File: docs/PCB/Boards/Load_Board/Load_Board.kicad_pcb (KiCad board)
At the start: 2 copper layers, 108.1 x 74.8 mm, 114 parts, among them J1 Conn_02x04_Odd_Even, J10 LVL_OUT_3, J11 LVL_IN_4, J12 LVL_OUT_4, J13 LVL_IN_6, J14 LVL_OUT_6, J15 LVL_IN_5, J16 LVL_OUT_5, J2 Conn_02x04_Odd_Even, J21 R_IN, J22 R_OUT, J23 SW_IN, J24 SW_OUT, J25 Divider_1, J26 Divider_2, J27 BZ_IN, J28 BZ_OUT, J29 LED_IN, J3 Conn_01x06_Pin, J30 LED_OUT, J31 CRYSTAL_IN, J32 CRYSTAL_OUT, J33 T_1, J34 T_2, J35 L_IN, J36 L_OUT, J37 C_IN, J38 C_OUT, J39 RV1, J4 Conn_01x06_Pin, J40 RV2, J41 RV3, J5 LVL_IN_2, J6 LVL_OUT_2, J7 LVL_IN_1, J8 LVL_OUT_1, J9 LVL_IN_3, Q1 BSS138, Q2 BSS138, Q3 BSS138, Q4 BSS138, Q5 BSS138, Q6 BSS138, Q7 BSS138, Q8 BSS138, SW1 Tact Switch 6x6mm / 13mm, U1 NE555P, Y1 Crystal, Y2 Crystal, Y3 Crystal

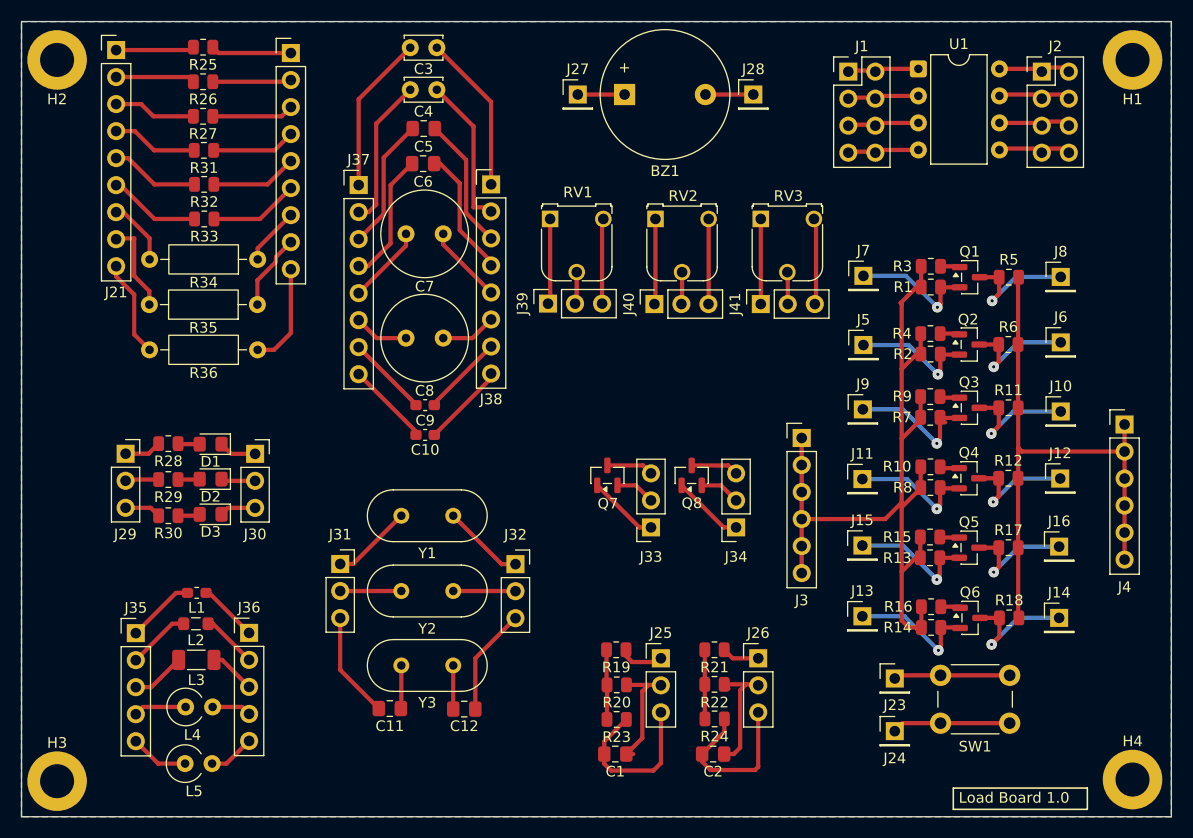
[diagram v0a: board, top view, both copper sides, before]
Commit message: Code review
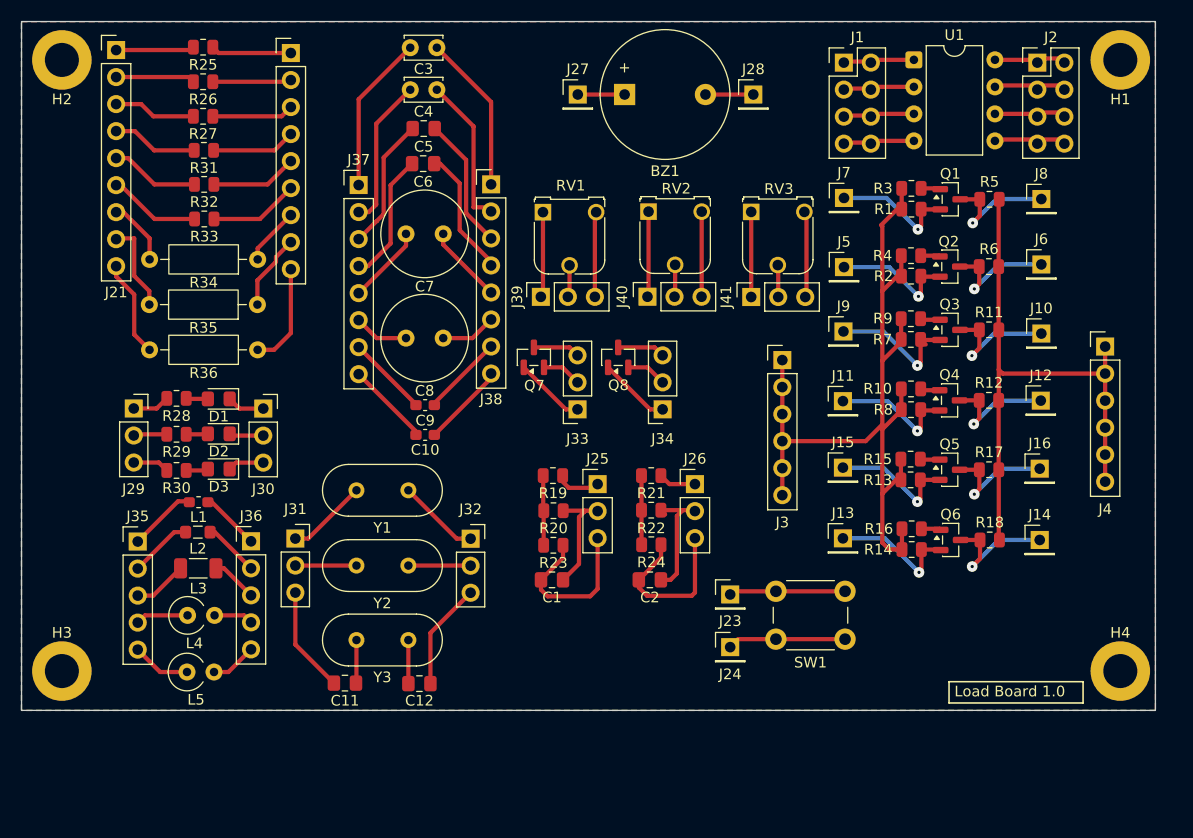
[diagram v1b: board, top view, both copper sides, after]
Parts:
- moved C1 17.4 mm to (171.6, 109.9)
- moved J26 17.4 mm to (185.0, 100.9)
- moved R19 17.4 mm to (171.7, 100.1)
- moved R23 17.4 mm to (171.7, 106.7)
- moved R24 17.4 mm to (180.9, 106.6)
- moved C2 17.4 mm to (180.8, 109.9)
- moved J25 17.4 mm to (175.9, 100.9)
- moved R20 17.4 mm to (171.7, 103.4)
- moved R21 17.4 mm to (180.9, 100.1)
- moved R22 17.4 mm to (180.9, 103.4)
- moved J23 17.4 mm to (188.3, 111.3)
- moved J24 17.4 mm to (188.3, 116.2)
- moved SW1 17.4 mm to (192.6, 111.0)
- moved J33 13.1 mm to (174.0, 93.9)
- moved J34 13.1 mm to (182.0, 93.9)
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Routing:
- net Divider_GND_1: track 11.2 -> 10.6 mm
- net Divider_IN_1: track 4.32 -> 3.67 mm
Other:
- board size 108.1 x 74.8 mm -> 106.6 x 64.8 mm
